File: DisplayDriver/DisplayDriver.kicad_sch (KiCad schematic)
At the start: 74 parts, among them SW1 KMR2, SW2 KMR2, U1 ESP32-S3-WROOM, U10 74AHCT245, U2 74AHCT245, U3 74AHCT245, U4 AP2112K-3.3, U5 ESP32-WROVER-B, U6 CH340N, U7 CP2102N-Axx-xQFN24, U8 ESP32-WROVER-B, U9 74AHCT245, X1 USB TYPE C

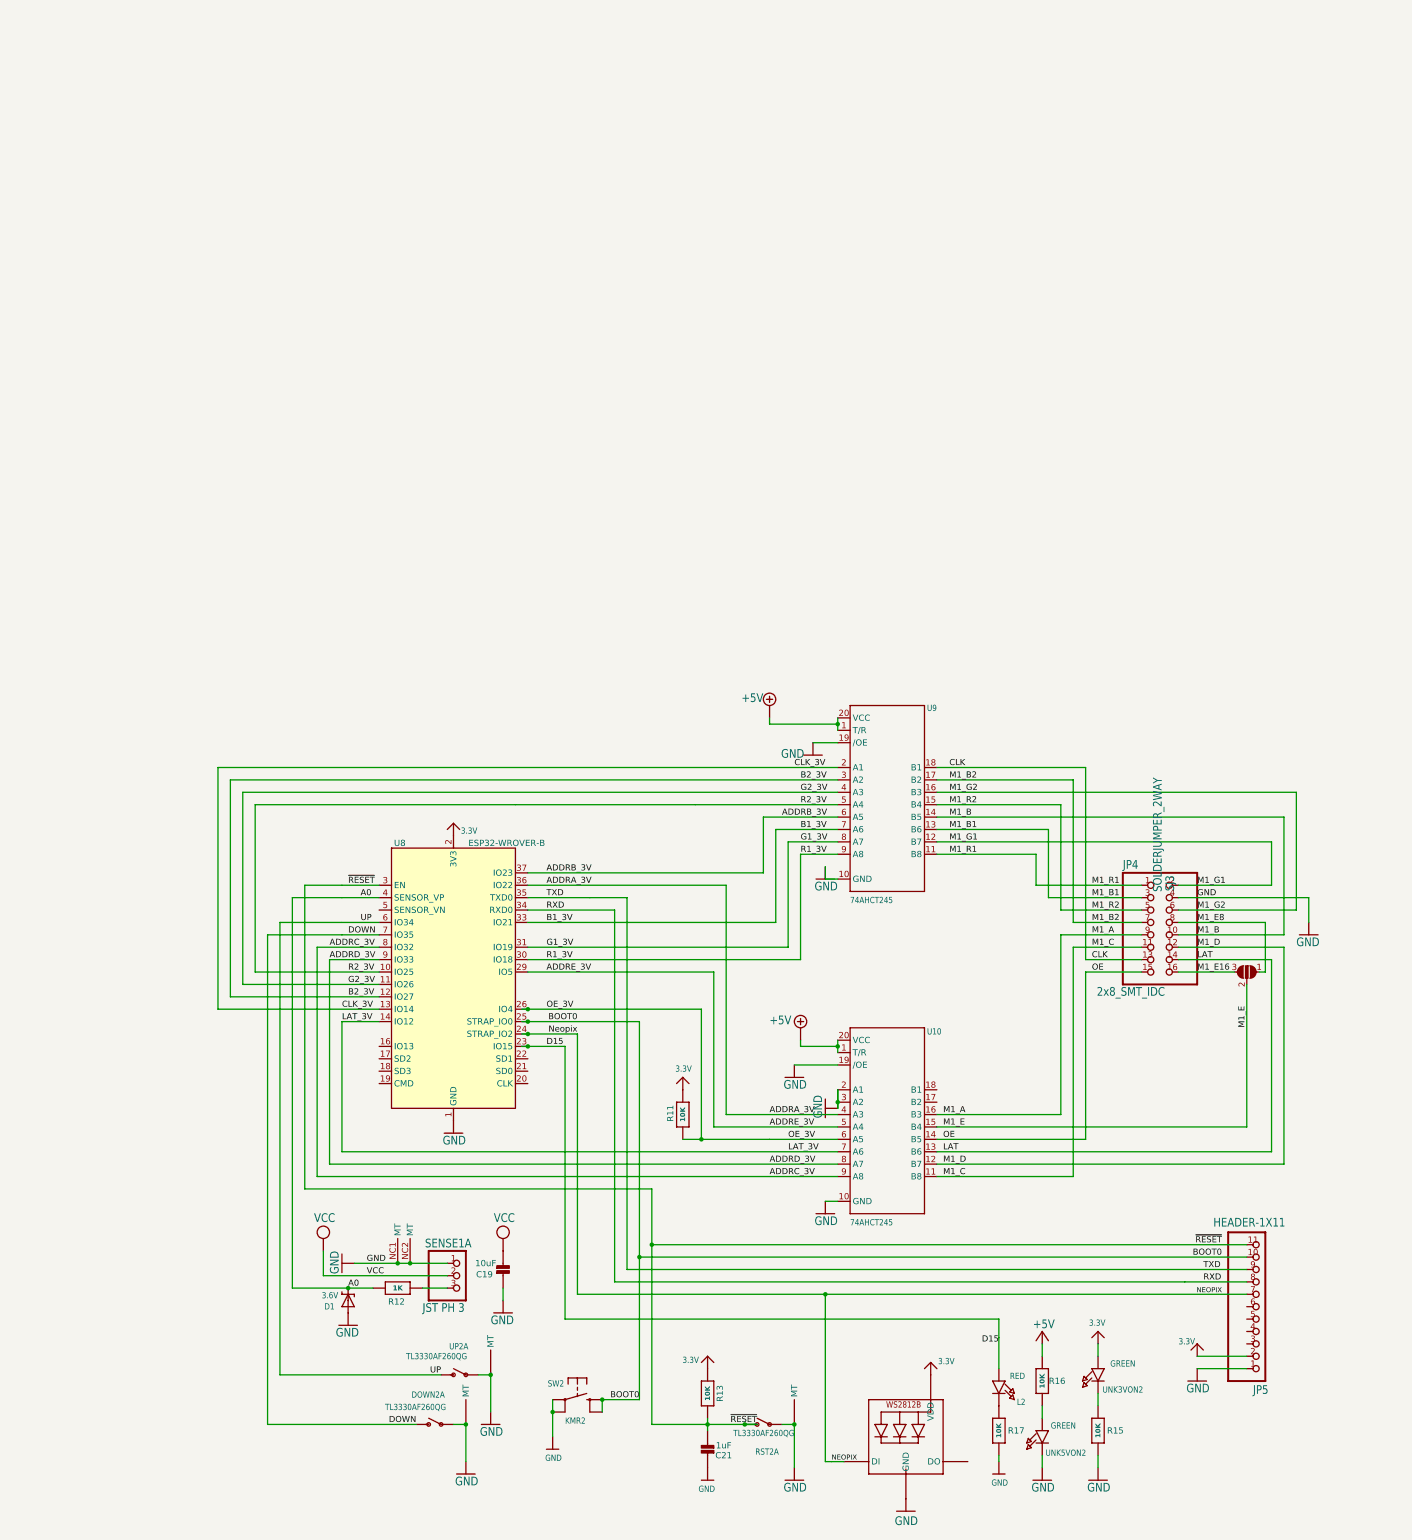
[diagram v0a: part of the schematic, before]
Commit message: final
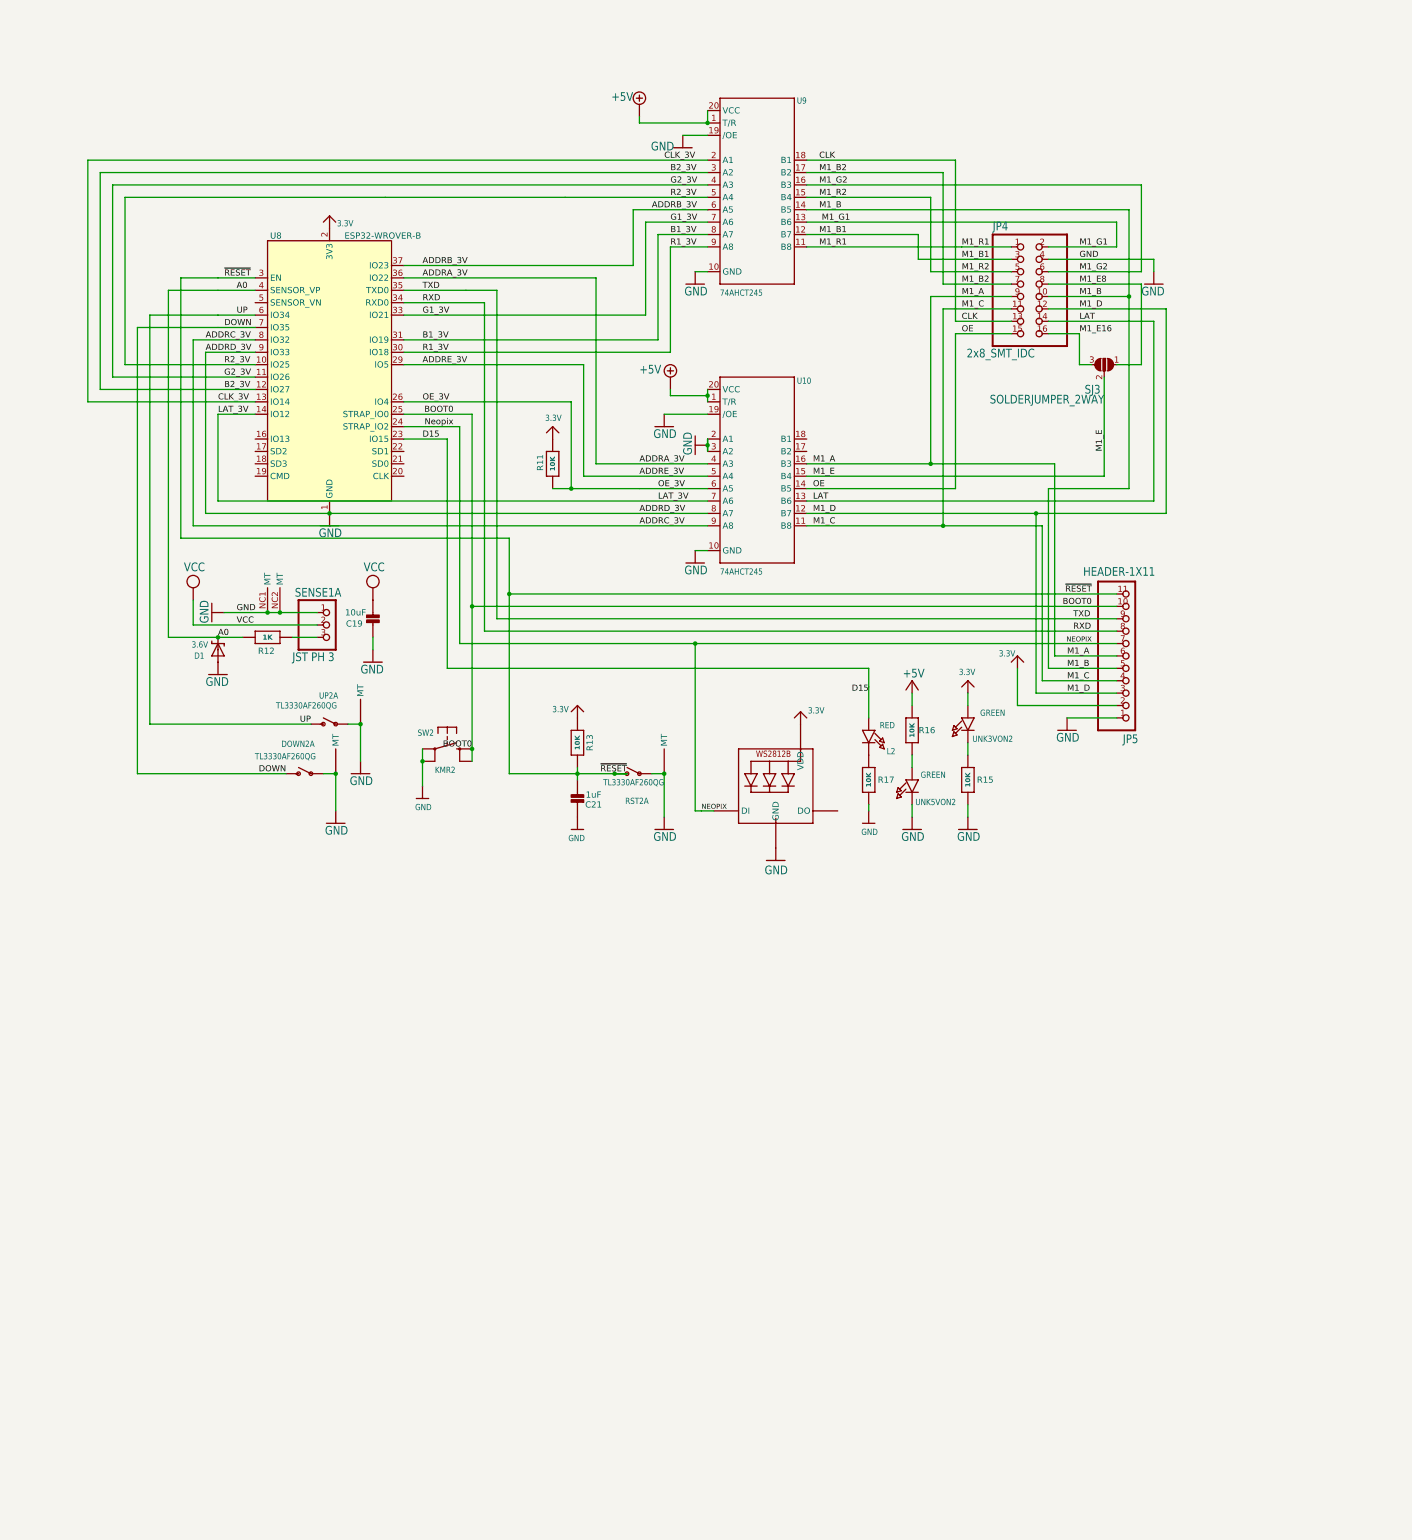
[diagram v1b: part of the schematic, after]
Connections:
- net ADDRD_3V is gone; now on net GND: U10.8 (A7), U3.4 (A3), U5.9 (IO33), U8.9 (IO33)
- net B1_3V: now also U8.31 (IO19), U9.8 (A7); no longer U8.33 (IO21), U9.7 (A6)
- net G1_3V: now also U8.33 (IO21), U9.7 (A6); no longer U8.31 (IO19), U9.8 (A7)
- net M1_A: now also JP5.6
- net M1_B: now also JP5.5
- net M1_B1: now also U9.12 (B7); no longer U9.13 (B6)
- net M1_C: now also JP5.4
- net M1_D: now also JP5.3
- net M1_G1: now also U9.13 (B6); no longer U9.12 (B7)
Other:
- moved on the sheet: C19, C21, D1, DOWN2A, JP4, JP5, L2, R11, R12, R13, R15, R16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
